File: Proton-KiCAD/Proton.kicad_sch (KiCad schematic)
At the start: 44 parts, among them J1 USB_C_Receptacle_USB2.0_14P, J9 Conn_01x03_Pin, SW1 BOOTSEL, SW2 RESET, U1 W25Q128JVS, U2 USBLC6-2P6, U3 NCP1117-3.3_SOT223, U4 RP2350_80QFN, Y1 ABM8-272-T3

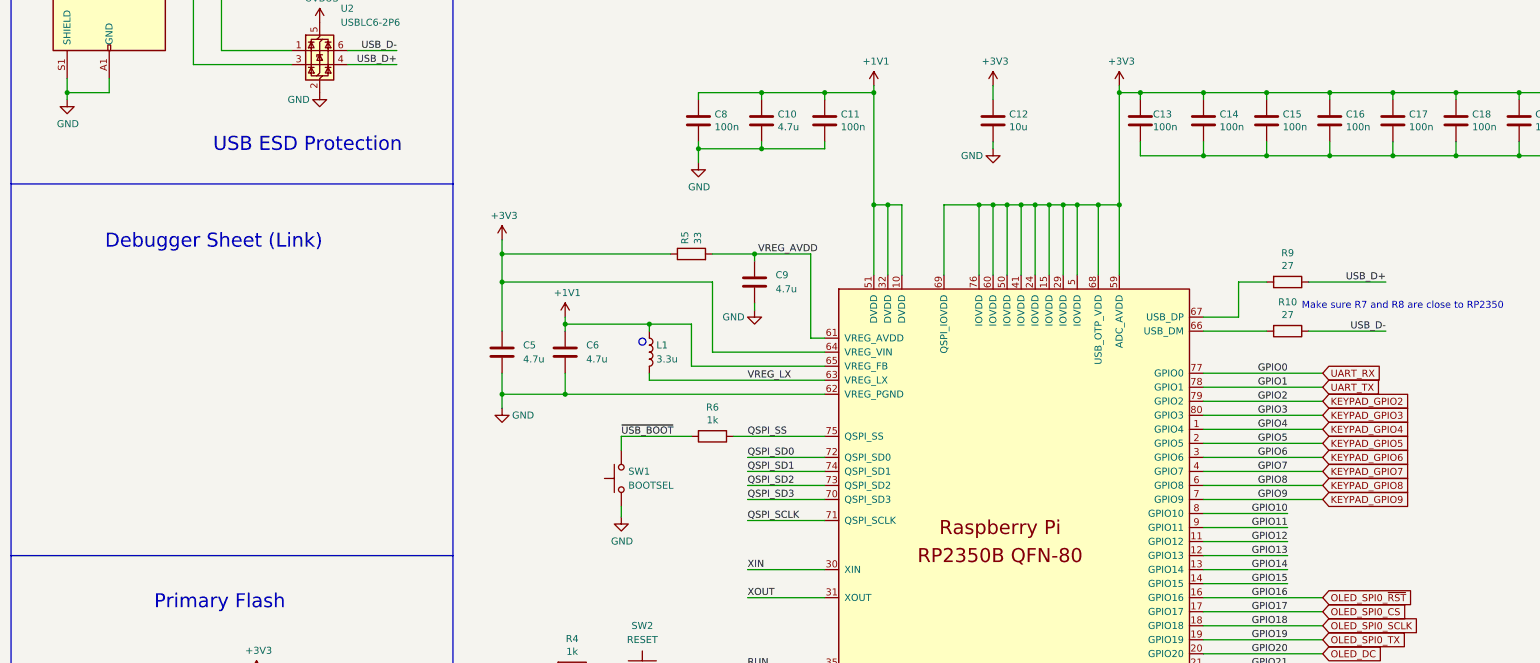
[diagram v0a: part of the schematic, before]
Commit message: ready for final check
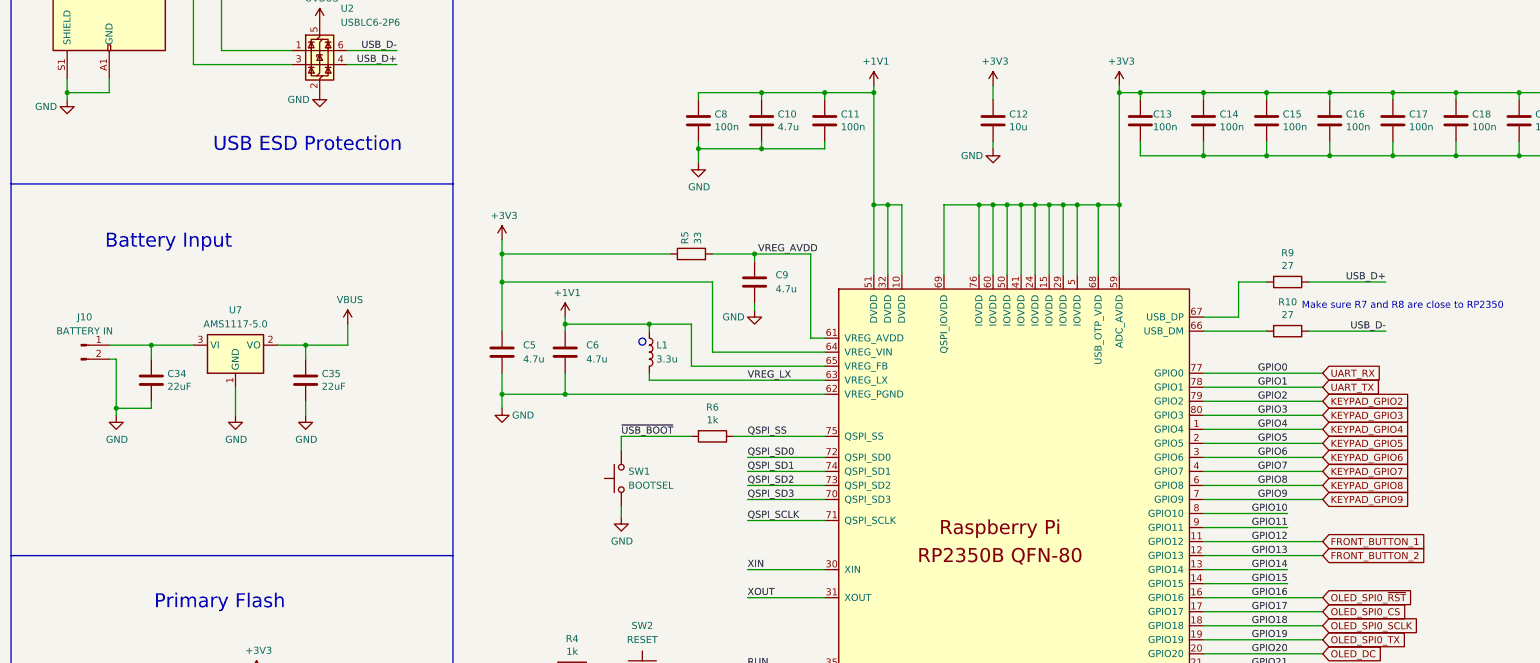
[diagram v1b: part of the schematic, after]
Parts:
- added C34, C35: 22uF, Capacitor_SMD:C_0805_2012Metric, symbol Device:C
- added J10: BATTERY IN, Connector_PinHeader_2.54mm:PinHeader_1x02_P2.54mm_Vertical, symbol Connector:Conn_01x02_Pin
- added U7: AMS1117-5.0, Package_TO_SOT_SMD:SOT-223-3_TabPin2, symbol Regulator_Linear:AMS1117-5.0
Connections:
- net GND: now also C34.2, C35.2, J10.2 (Pin_2), U7.1 (GND)
- net VBUS: now also C35.1, U7.2 (VO)
- net GPIO12 renamed FRONT_BUTTON_1
- net GPIO13 renamed FRONT_BUTTON_2
- new net: C34.1, J10.1 (Pin_1), U7.3 (VI)
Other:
- note added: "Battery Input"
- note removed: "Debugger Sheet (Link)"
